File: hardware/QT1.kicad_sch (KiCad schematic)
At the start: 13 parts, among them M1 OSHW-LOGO, U1 TLE2141CD, U2 AD8561ARZ, U3 MCP601-xOT, U4 Teensy 4.0

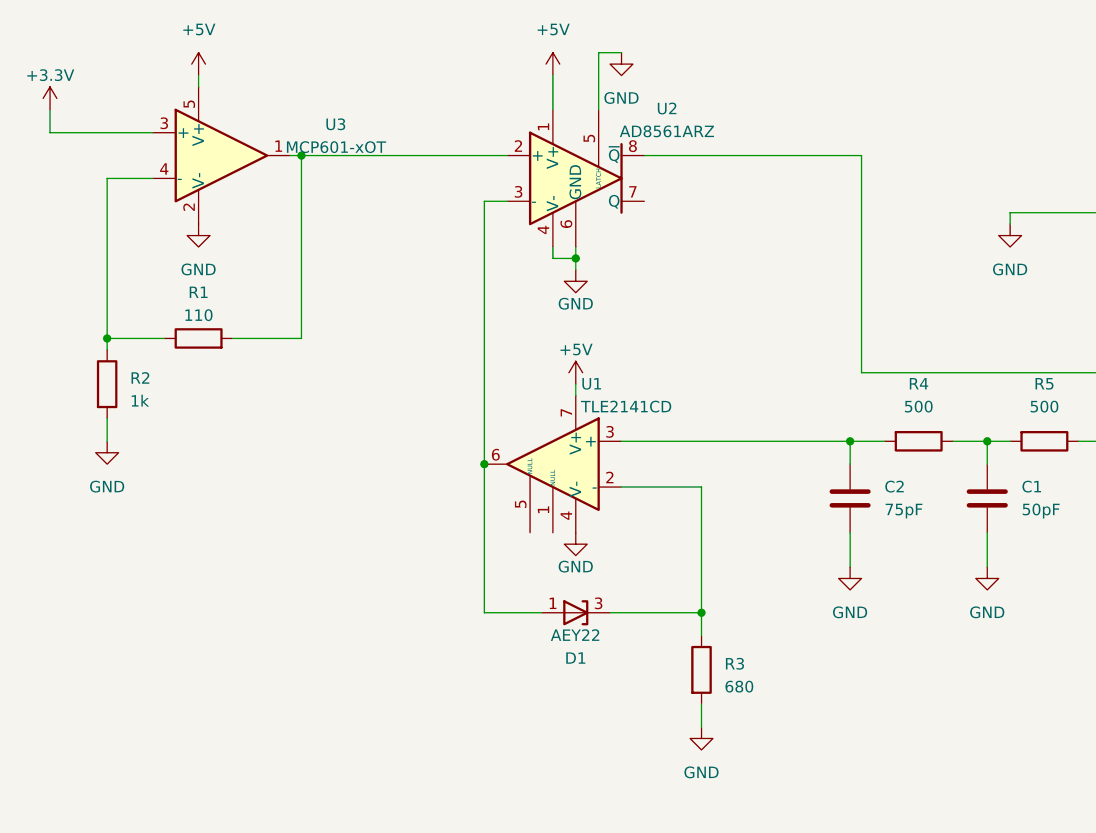
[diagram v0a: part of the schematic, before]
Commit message: Add files via upload
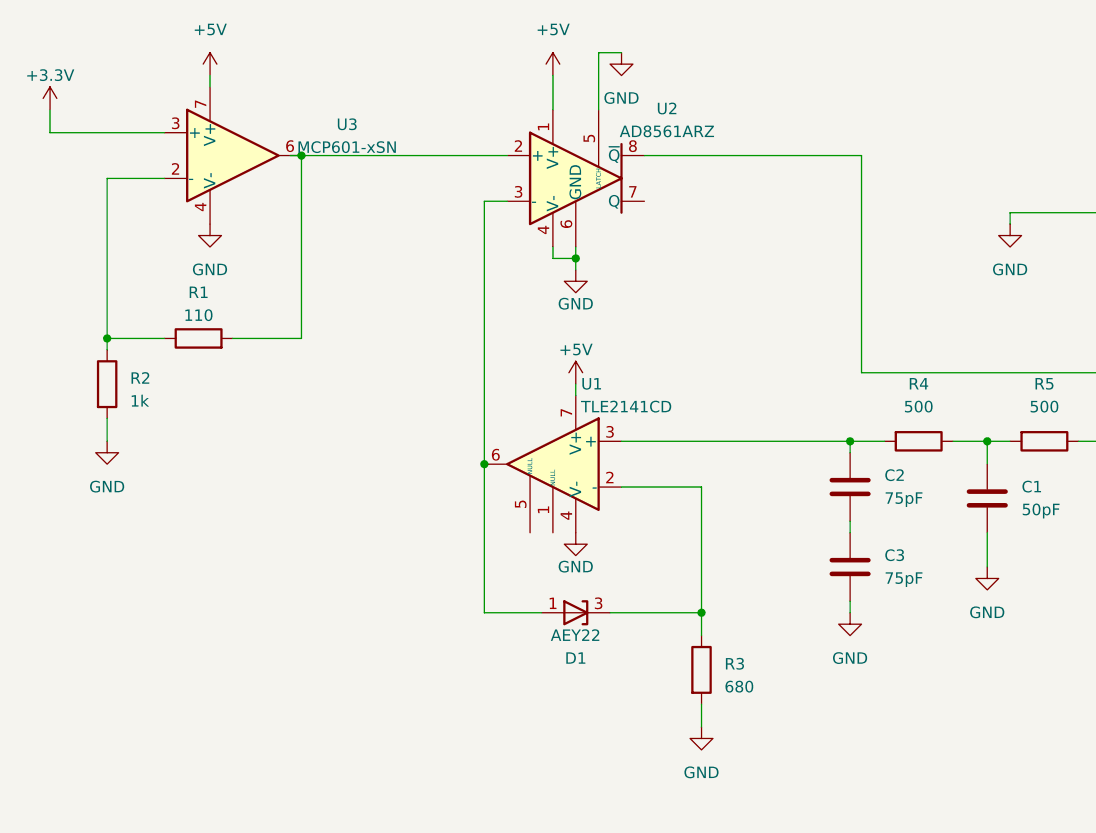
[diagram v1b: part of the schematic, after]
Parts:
- removed U3: MCP601-xOT, Package_TO_SOT_SMD:SOT-23-5, symbol Amplifier_Operational:MCP601-xOT
- added C3: 75pF, Capacitor_SMD:C_0603_1608Metric, symbol Device:C
- added U3: MCP601-xSN, Package_SO:SOIC-8_3.9x4.9mm_P1.27mm, symbol Amplifier_Operational:MCP601-xSN
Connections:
- net +3.3V: now also U3.3 (+)
- net +5V: now also U3.7 (V+)
- net GND1: now also C3.2; no longer C2.2
- net GND3: now also U3.4 (V-)
- net at R1.1, R2.1: now also U3.2 (-)
- net at R1.2, U2.2 (+): now also U3.6
- new net: C2.2, C3.1
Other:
- moved on the sheet: C2
